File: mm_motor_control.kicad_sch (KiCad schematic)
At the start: 0 parts

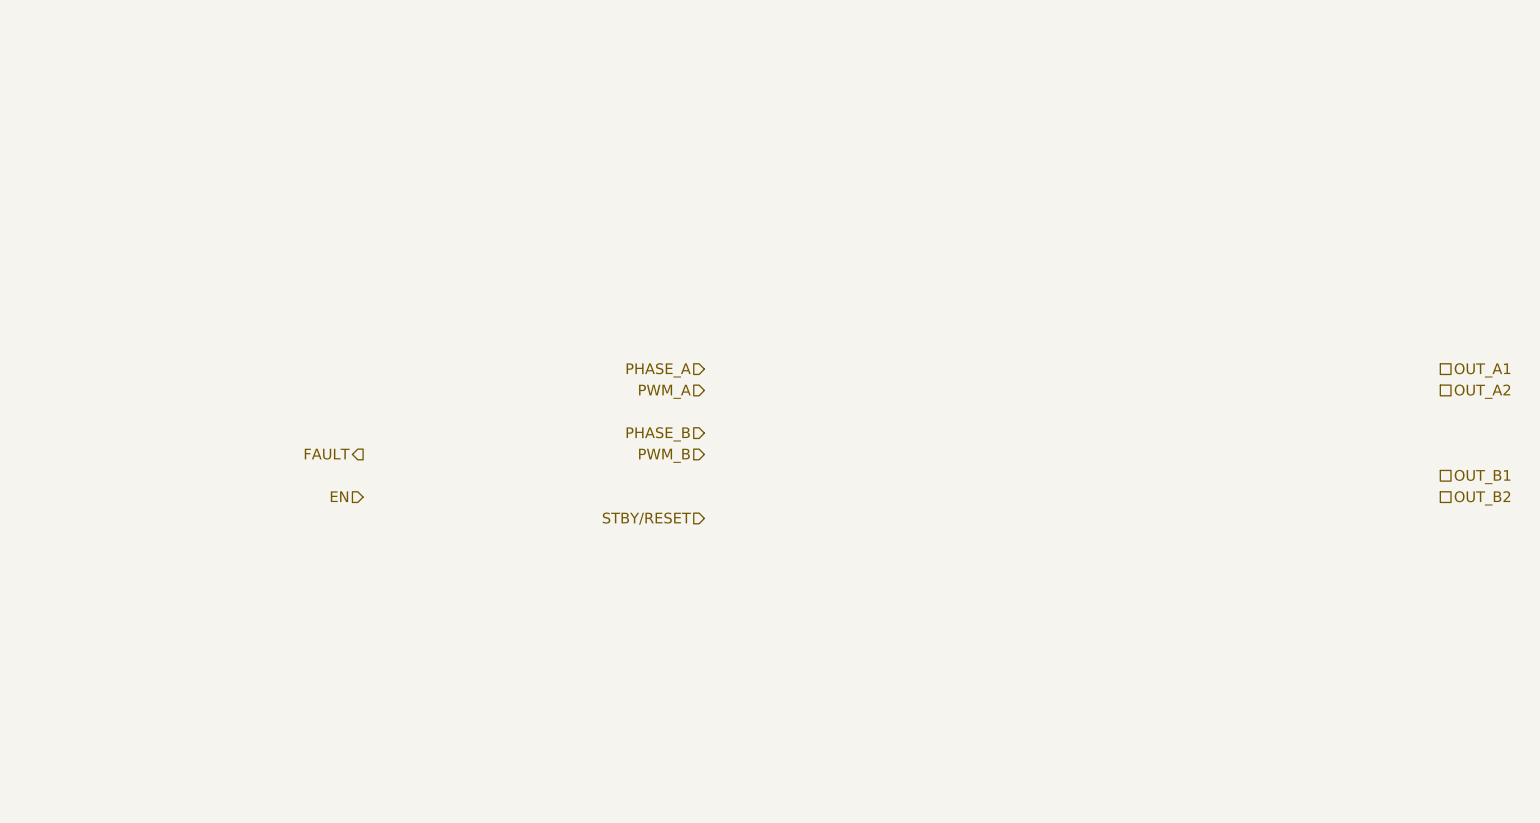
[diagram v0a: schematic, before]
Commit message: tp2
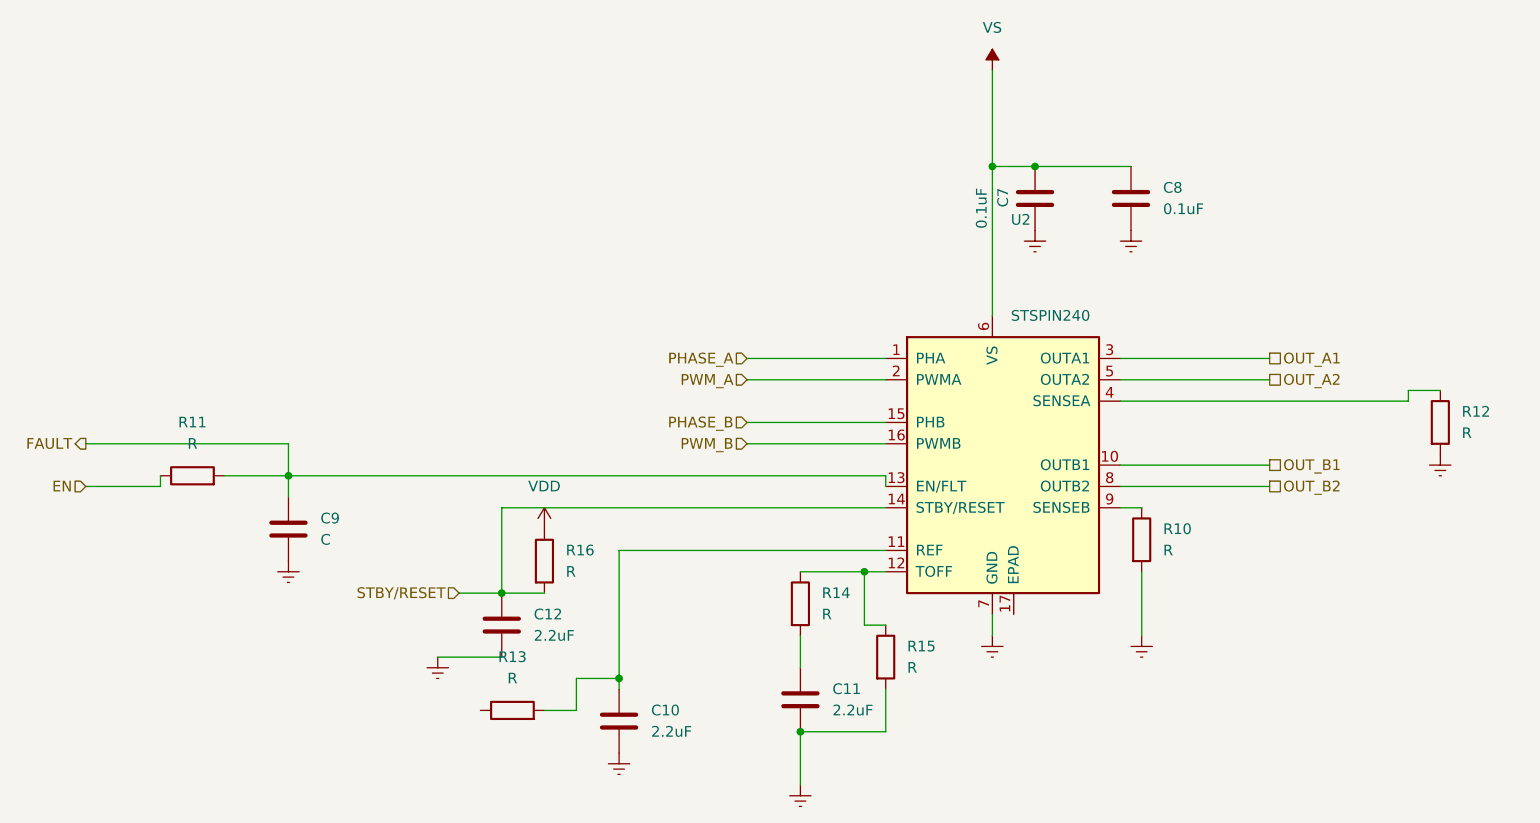
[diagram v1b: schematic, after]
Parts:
- added C10, C11, C12: 2.2uF, symbol Device:C
- added C7, C8: 0.1uF, symbol Device:C
- added C9: C, symbol Device:C
- added R10, R11, R12, R13, R14, R15, R16: R, symbol Device:R
- added U2: STSPIN240, Package_DFN_QFN:VQFN-16-1EP_3x3mm_P0.5mm_EP1.8x1.8mm, symbol Driver_Motor:STSPIN240
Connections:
- net EN: now also R11.1
- net FAULT: now also C9.1, R11.2, U2.13 (EN/FLT)
- net OUT_A1: now also U2.3 (OUTA1)
- net OUT_A2: now also U2.5 (OUTA2)
- net OUT_B1: now also U2.10 (OUTB1)
- net OUT_B2: now also U2.8 (OUTB2)
- net PHASE_A: now also U2.1 (PHA)
- net PHASE_B: now also U2.15 (PHB)
- net PWM_A: now also U2.2 (PWMA)
- net PWM_B: now also U2.16 (PWMB)
- net STBY/RESET: now also C12.1, R16.2, U2.14 (STBY/RESET)
- new net: C11.2, R14.2
- new net: R10.1, U2.9 (SENSEB)
- new net: R12.1, U2.4 (SENSEA)
- new net: C10.1, R13.2, U2.11 (REF)
- new net: R14.1, R15.1, U2.12 (TOFF)
- new net Earth: C10.2, C11.1, C12.2, C7.1, C8.1, C9.2, R10.2, R12.2, R15.2, U2.7 (GND)
- new net VDD: R16.1
- new net VS: C7.2, C8.2, U2.6 (VS)
